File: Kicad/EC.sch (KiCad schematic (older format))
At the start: 18 parts, among them U1 MCP6244

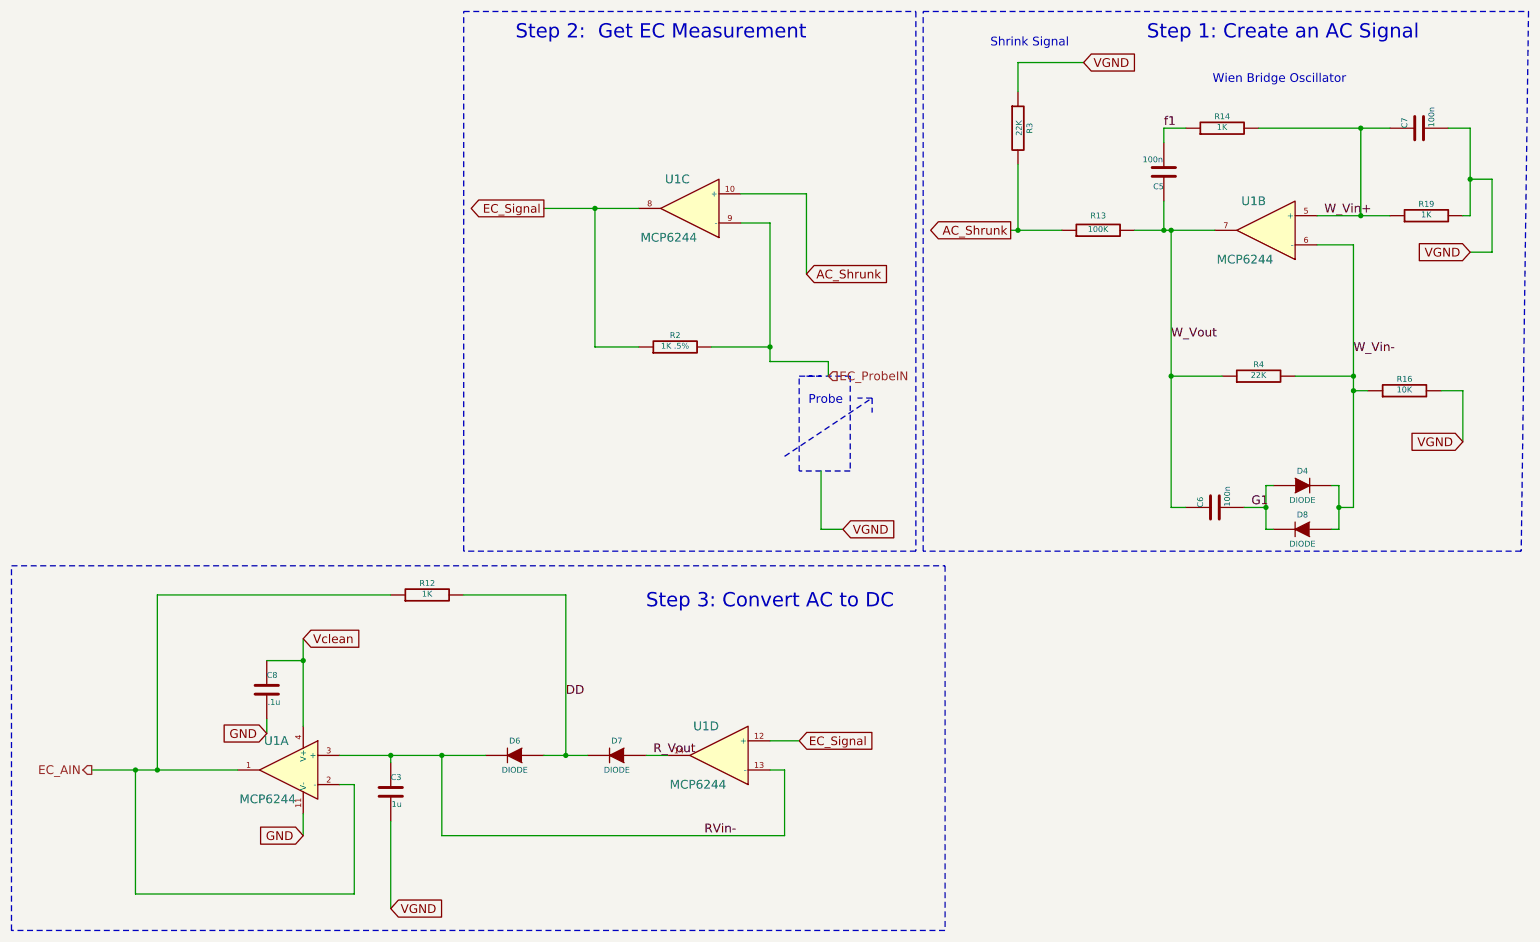
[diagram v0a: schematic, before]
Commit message: changes to layout after 12/22/2014 helpout
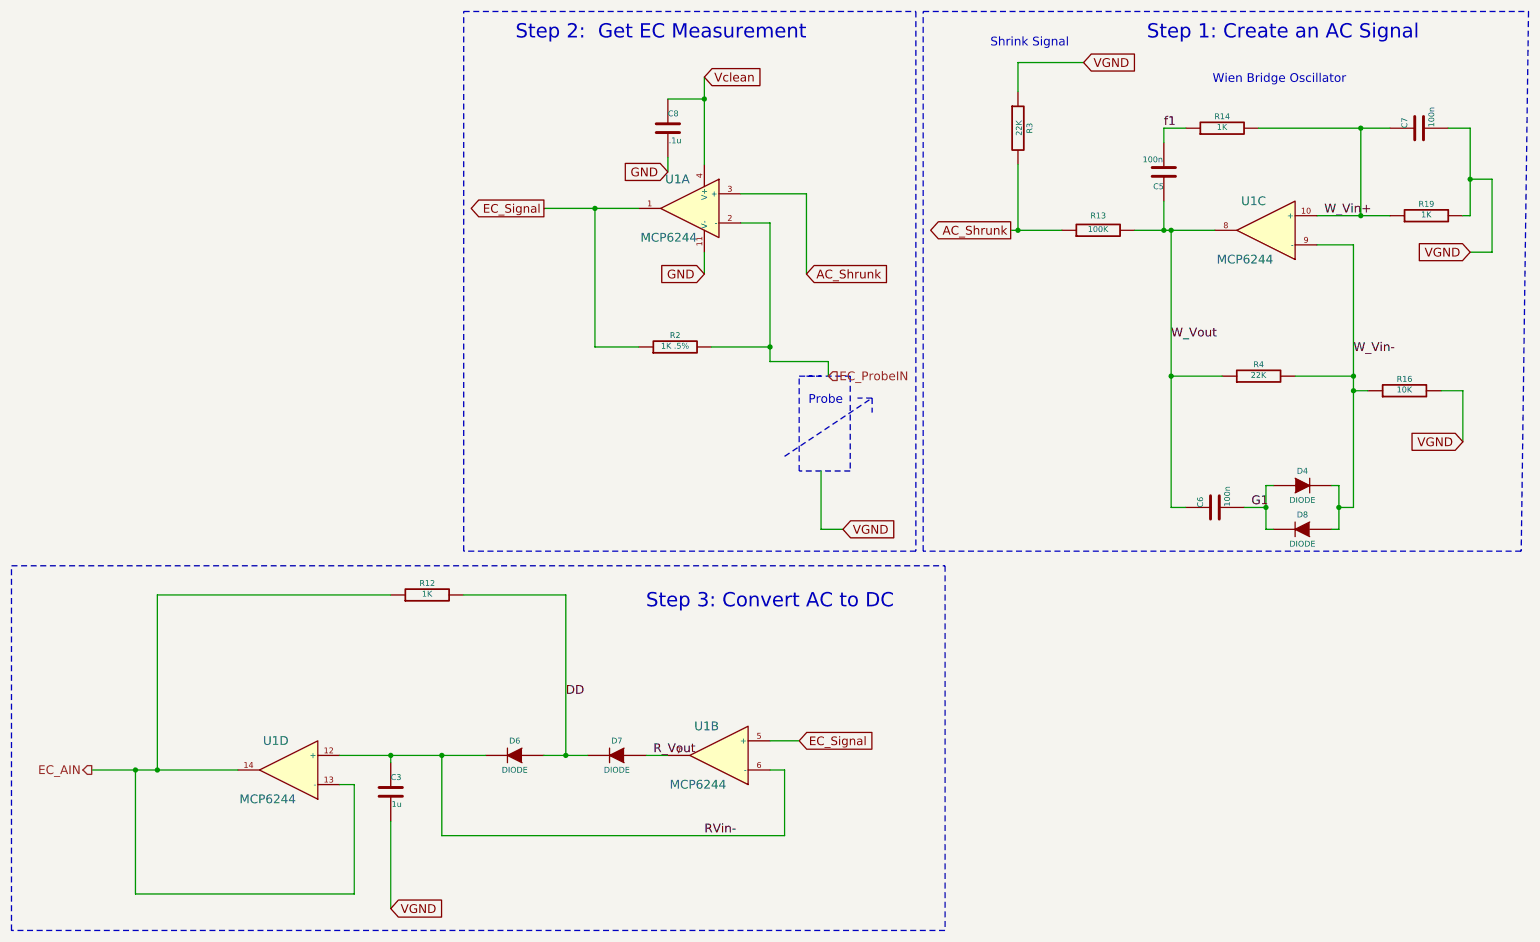
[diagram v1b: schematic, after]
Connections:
- net AC_Shrunk: now also U1.3 (+); no longer U1.10 (+)
- net EC_AIN: now also U1.13 (-), U1.14; no longer U1.1, U1.2 (-)
- net EC_ProbeIN: now also U1.2 (-); no longer U1.9 (-)
- net EC_Signal: now also U1.1, U1.5 (+); no longer U1.12 (+), U1.8
- net GND: now also U1.11 (V-); no longer U1.11 (V-)
- net RVin-: now also U1.12 (+), U1.6 (-); no longer U1.13 (-), U1.3 (+)
- net R_Vout: now also U1.7; no longer U1.14
- net Vclean: now also U1.4 (V+); no longer U1.4 (V+)
- net W_Vin+: now also U1.10 (+); no longer U1.5 (+)
- net W_Vin-: now also U1.9 (-); no longer U1.6 (-)
- net W_Vout: now also U1.8; no longer U1.7
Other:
- moved on the sheet: C8
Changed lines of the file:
@@
 Sheet 5 8
 Title ""
-Date "20 dec 2014"
+Date "23 dec 2014"
 Rev ""
 Comp ""
@@
 $Comp
 L MCP6244 U1
-U 2 1 5419C202
+U 3 1 5419C202
 P 9500 2300
 F 0 "U1" H 9600 2500 60  0000 L CNN
@@
 F 2 "~" H 9600 2300 60  0000 C CNN
 F 3 "~" H 9600 2300 60  0000 C CNN
-	2    9500 2300
+	3    9500 2300
 	-1   0    0    -1
 $EndComp
 $Comp
 L MCP6244 U1
-U 3 1 5419C208
+U 1 1 5419C208
 P 5550 2150
 F 0 "U1" H 5650 2350 60  0000 L CNN
@@
 F 2 "~" H 5650 2150 60  0000 C CNN
 F 3 "~" H 5650 2150 60  0000 C CNN
-	3    5550 2150
+	1    5550 2150
 	-1   0    0    -1
 $EndComp
 $Comp
 L MCP6244 U1
-U 4 1 5419C20E
+U 2 1 5419C20E
 P 5750 5900
 F 0 "U1" H 5850 6100 60  0000 L CNN
@@
 F 2 "~" H 5850 5900 60  0000 C CNN
 F 3 "~" H 5850 5900 60  0000 C CNN
-	4    5750 5900
+	2    5750 5900
 	-1   0    0    -1
 $EndComp
@@
 L C C8
 U 1 1 548611AE
-P 2550 5450
-F 0 "C8" H 2550 5550 40  0000 L CNN
-F 1 ".1u" H 2556 5365 40  0000 L CNN
-F 2 "~" H 2588 5300 30  0000 C CNN
-F 3 "~" H 2550 5450 60  0000 C CNN
-	1    2550 5450
+P 5300 1600
+F 0 "C8" H 5300 1700 40  0000 L CNN
+F 1 ".1u" H 5306 1515 40  0000 L CNN
+F 2 "~" H 5338 1450 30  0000 C CNN
+F 3 "~" H 5300 1600 60  0000 C CNN
+	1    5300 1600
 	1    0    0    -1
 $EndComp
 Wire Wire Line
-	2800 5100 2800 5700
-Wire Wire Line
-	2550 5250 2800 5250
-Connection ~ 2800 5250
+	5550 1250 5550 1850
+Wire Wire Line
+	5300 1400 5550 1400
+Connection ~ 5550 1400
 Wire Notes Line
 	800  4600 7200 4600
@@
 Connection ~ 1650 6000
 Wire Wire Line
-	2550 5650 2550 5750
-Wire Wire Line
-	2800 6300 2800 6450
-Text GLabel 2800 5100 2    60   Input ~ 0
+	5300 1800 5300 1900
+Wire Wire Line
+	5550 2450 5550 2600
+Text GLabel 5550 1250 2    60   Input ~ 0
 Vclean
-Text GLabel 2800 6450 0    60   Input ~ 0
+Text GLabel 5550 2600 0    60   Input ~ 0
 GND
 Text GLabel 3400 6950 2    60   Input ~ 0
@@
 $Comp
 L MCP6244 U1
-U 1 1 549068E6
+U 4 1 549068E6
 P 2800 6000
 F 0 "U1" H 2900 6200 60  0000 L CNN
@@
 F 2 "~" H 2900 6000 60  0000 C CNN
 F 3 "~" H 2900 6000 60  0000 C CNN
-	1    2800 6000
-	-1   0    0    -1
-$EndComp
-Text GLabel 2550 5750 0    60   Input ~ 0
+	4    2800 6000
+	-1   0    0    -1
+$EndComp
+Text GLabel 5300 1900 0    60   Input ~ 0
 GND
 $EndSCHEMATC
